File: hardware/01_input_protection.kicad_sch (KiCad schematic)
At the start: 22 parts, among them J1 USB4105-GF-A, Q1 MMBT3906, U1 CH224K, U2 TPS26600PWPR

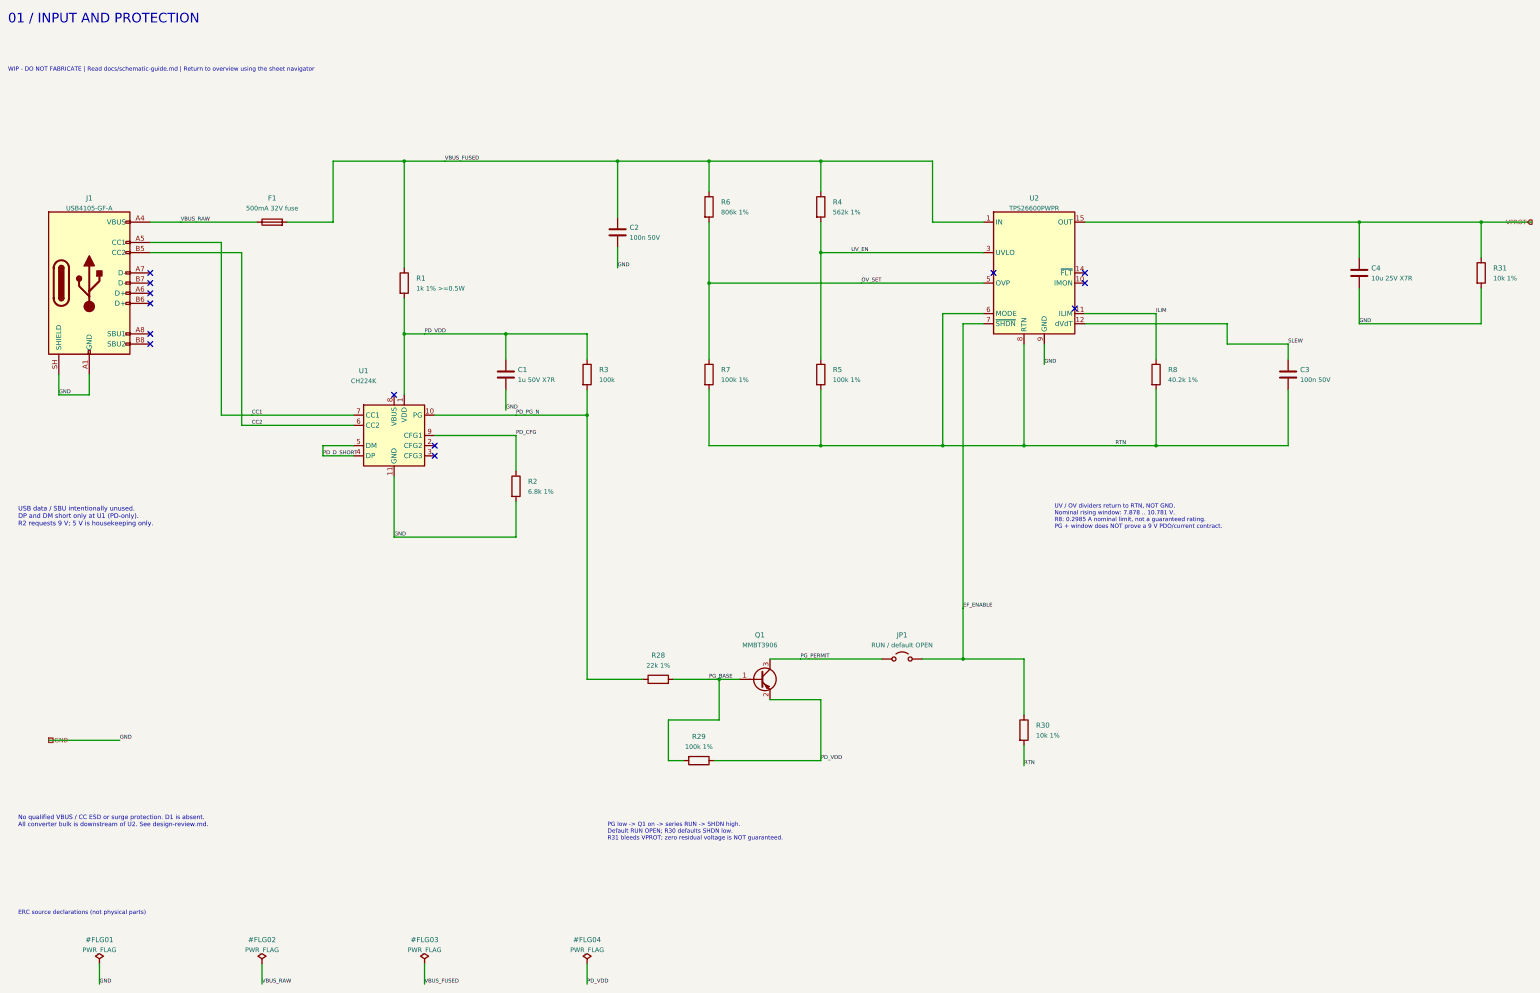
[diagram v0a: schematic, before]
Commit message: Update on the PCB.
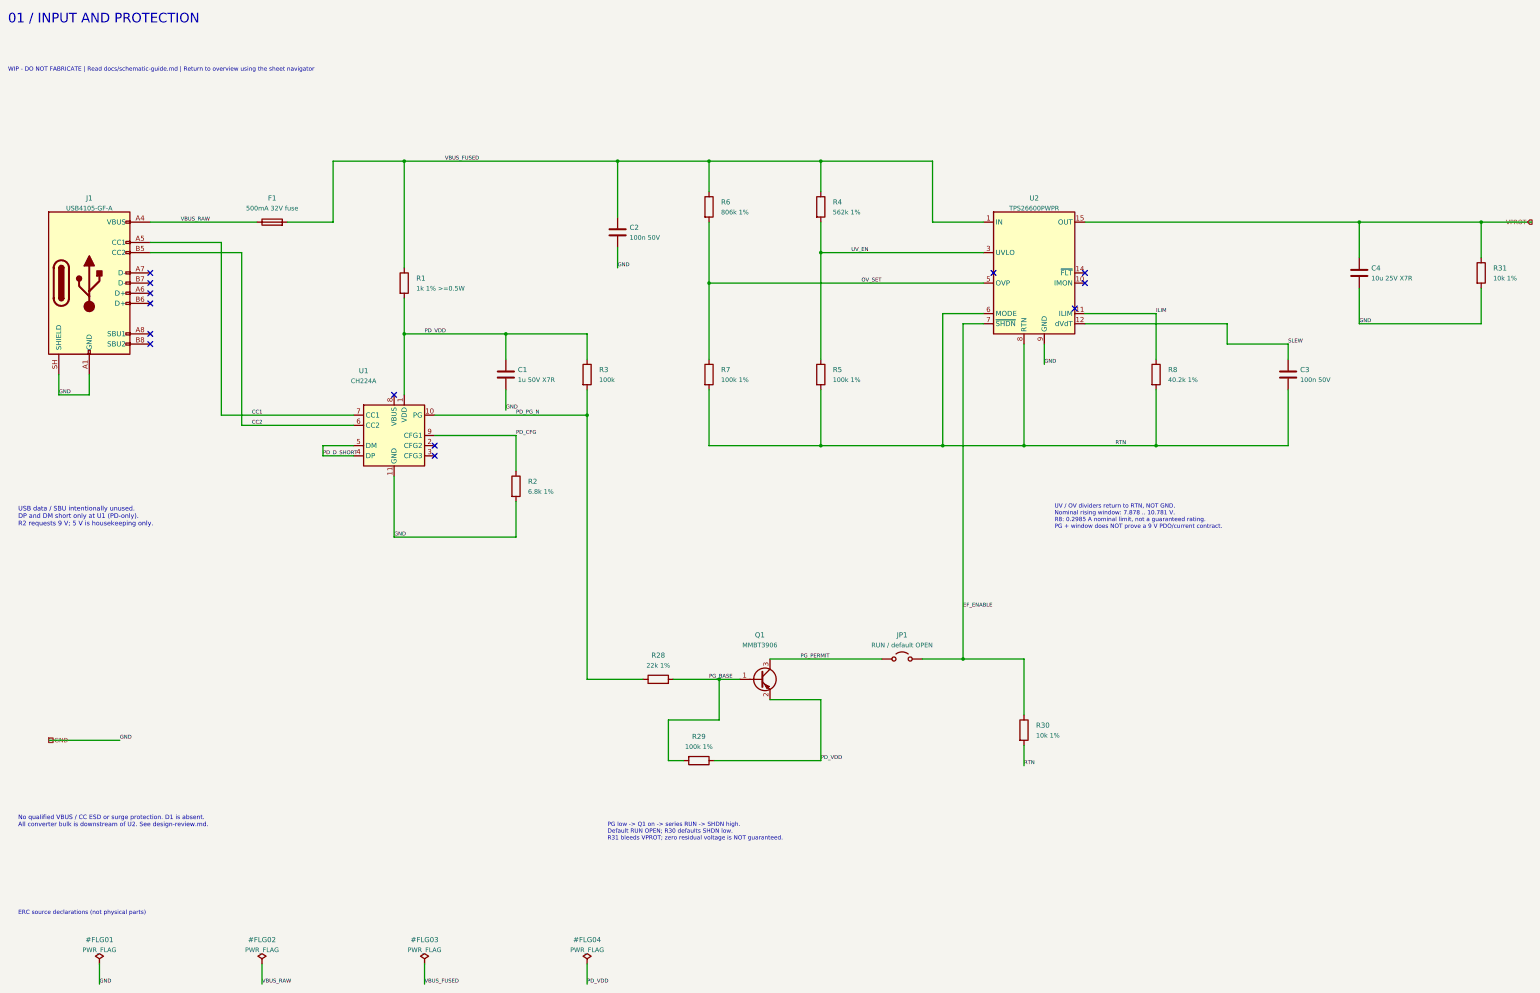
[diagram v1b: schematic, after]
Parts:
- U1: value CH224K -> CH224A
